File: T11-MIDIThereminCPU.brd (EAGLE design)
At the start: 102.5 x 53.3 mm, 66 parts, among them IC1 UA78M05DCY, IC4 QUAD_OPAMPD, IC5 4069D, J1 DCJ0202, Q1 16MHz, U1 ATMEGA328P-AU

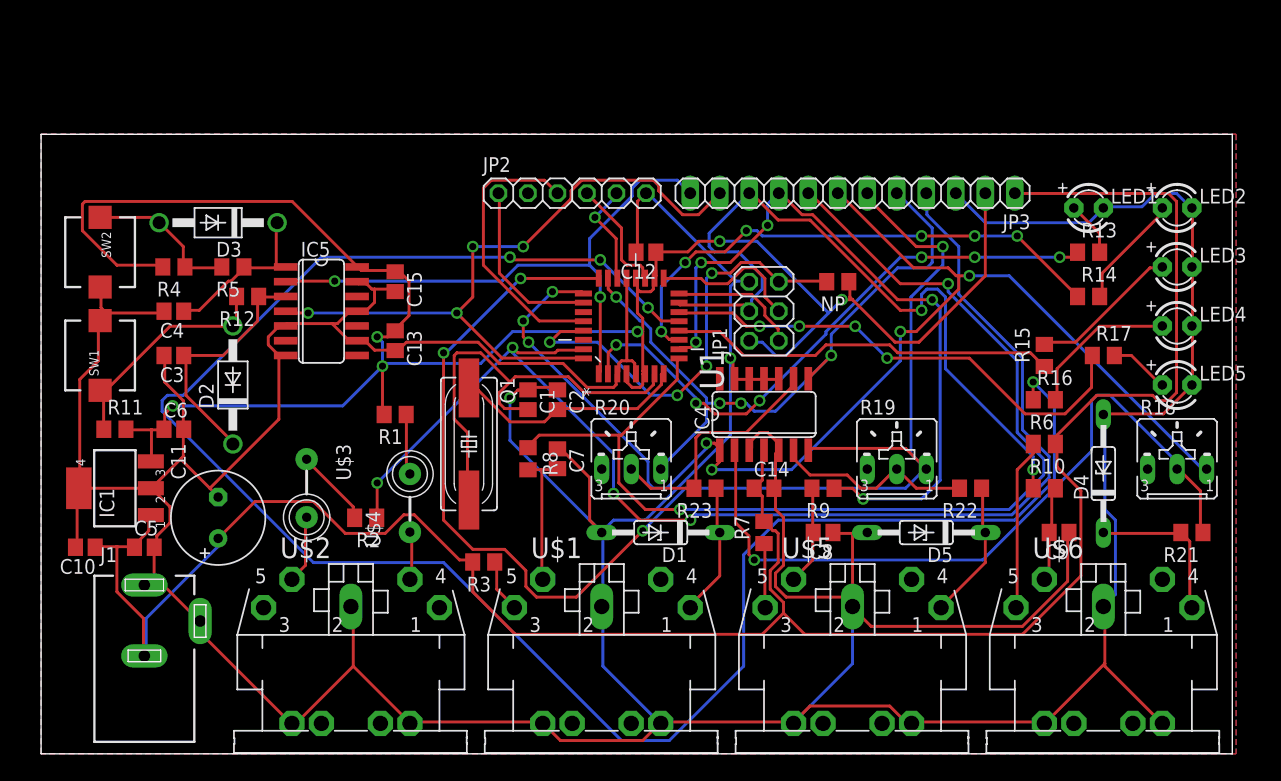
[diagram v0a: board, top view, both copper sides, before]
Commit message: Add files via upload
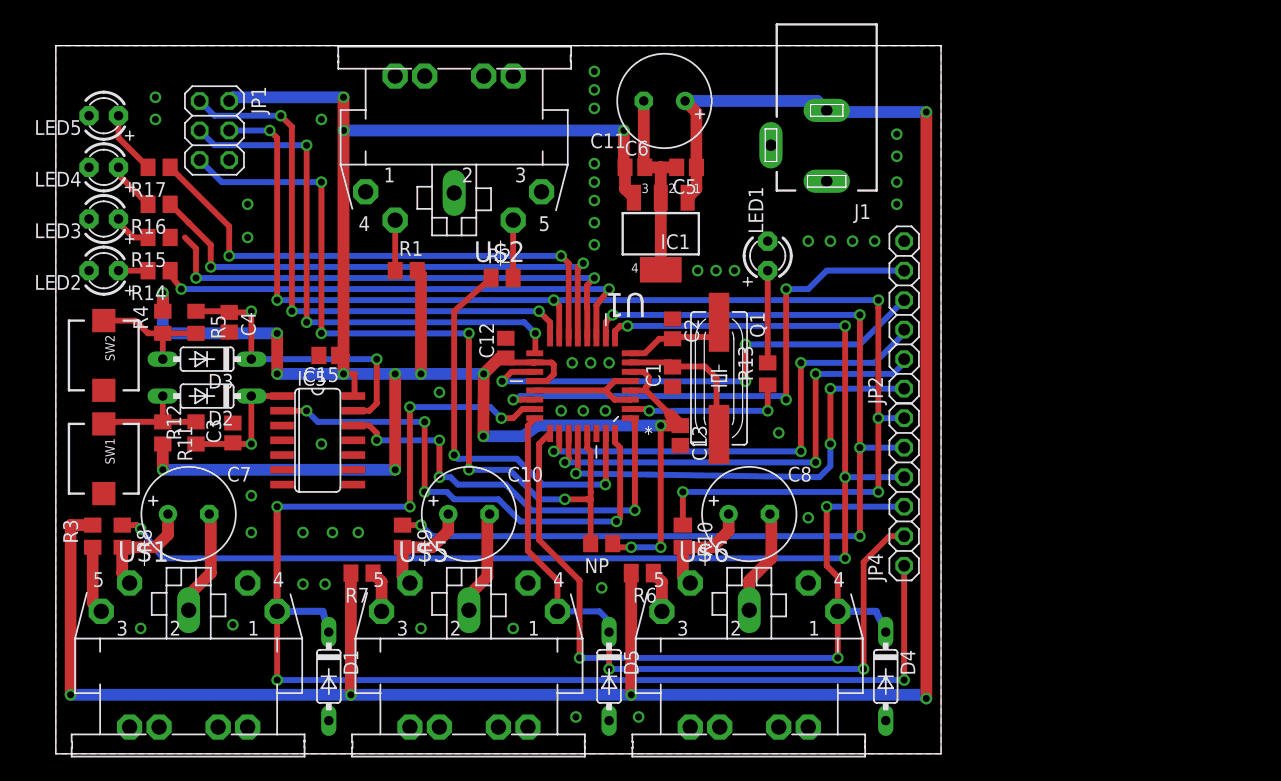
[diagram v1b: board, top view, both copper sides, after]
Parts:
- removed C14: 0.1u, adafruit:C0805
- removed C9: 100n, adafruit:C0805
- removed IC4: QUAD_OPAMPD, adafruit:SO14
- removed JP3: (no value), adafruit:1X12
- removed R18, R19, R20: 10k, pot:B25U
- removed R21, R22, R23: 1k, resistor:R0805
- removed U$3, U$4: 1k@100MHz, adafruit:FB
- added JP4: (no value), adafruit:1X06
- C10: value 0.1u -> 100uF; device adafruit:C0805 -> adafruit:E3,5-8
- C7, C8: value 100n -> 100uF; device adafruit:C0805 -> adafruit:E3,5-8
- D1, D4, D5: device diode:DO35Z10 -> diode:DO35-7
- D2, D3: value 1N4004 -> 1N4148DO35-7; device diode:DO41-10 -> diode:DO35-7
- R10, R8, R9: value 1k -> 100
- moved LED5 95.3 mm to (4.13, 54.9), turned to 180 degrees
- moved LED4 93.4 mm to (4.13, 50.5), turned to 180 degrees
- moved LED2 92.6 mm to (4.13, 41.6), turned to 180 degrees
- moved LED3 92.5 mm to (4.13, 46.0), turned to 180 degrees
- moved R17 82.9 mm to (8.89, 50.5), turned to 180 degrees
- moved R14 80.0 mm to (8.89, 41.6), turned to 180 degrees
- moved R16 78.0 mm to (8.89, 47.3), turned to 180 degrees
- moved R15 76.9 mm to (8.89, 44.5), turned to 180 degrees
- moved J1 71.6 mm to (66.4, 52.4), turned to 180 degrees
- moved U$2 61.6 mm to (34.3, 61.0), turned to 180 degrees
- moved C5 57.0 mm to (54.3, 50.5), turned to 180 degrees
- moved C11 52.6 mm to (52.4, 56.2), turned to 180 degrees
- moved IC1 51.8 mm to (52.1, 44.8), turned to 180 degrees
- moved JP1 49.8 mm to (13.7, 53.7), turned to 270 degrees
- moved C6 45.6 mm to (49.8, 50.5)
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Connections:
- removed net N$1: U$2.4, U$4.P$1
- removed net N$18: IC4.9, R20.S, R23.2
- removed net N$19: IC4.2, R18.S, R21.1
- removed net N$21: D1.C, R23.1, U$1.1
- removed net N$22: IC4.6, R19.S, R22.2
- removed net N$23: D4.C, R21.2, U$6.1
- removed net N$25: D5.C, R22.1, U$5.1
- removed net N$3: U$2.5, U$3.P$2
- net +12V: no longer C10.1, C14.1, IC4.4, JP3.1
- net +5V: no longer JP3.2
- net ANALOG_IN_1: now also D1.C, JP4.1, U$1.1; no longer IC4.8, JP3.5, R20.A
- net ANALOG_IN_2: now also D5.C, JP4.2, U$5.1; no longer IC4.7, JP3.6, R19.A
- net ANALOG_IN_3: now also D4.C, JP4.3, U$6.1; no longer IC4.1, JP3.7, R18.A
- net GND: now also C10.-, C7.-, C8.-, IC5.3; no longer C10.2, C14.2, C7.1, C8.1, C9.1, IC4.10, IC4.11, IC4.12, IC4.13, IC4.3, IC4.5, IC5.13, JP3.3
- net INT0: now also IC5.2; no longer IC5.4, JP3.11
- net INT1: now also IC5.12; no longer IC5.2, JP3.12
- net MOSI: now also JP4.6; no longer JP3.10
- net N$10: now also C10.+; no longer C8.2
- net N$13: now also U$2.5; no longer U$3.P$1
- net N$14: now also IC5.1; no longer IC5.3
- net N$2: now also U$2.4; no longer U$4.P$2
- net N$26: now also C7.+; no longer C7.2
- net N$5: now also C8.+; no longer C9.2
- net N$6: now also IC5.13; no longer IC5.1
- net PC3: now also JP2.3; no longer JP2.1
- net PC5: now also JP2.1; no longer JP2.3
- net SIGNAL_OUT_1: now also JP4.4; no longer JP3.8
- net SIGNAL_OUT_2: now also JP4.5; no longer JP3.9
- net TX: no longer JP3.4
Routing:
- net GND: track 485.2 -> 56.4 mm, vias 2 -> 48
- net LED_4: track 167.0 -> 46.4 mm, vias 4 -> 2
- net TX: track 110.8 -> 35.1 mm, vias 4 -> 2
- net N$19: track 64.4 -> 0.00 mm, vias 1 -> 0
- net ANALOG_IN_2: track 120.5 -> 62.4 mm, vias 4 -> 2
- net ANALOG_IN_1: track 57.9 -> 116.0 mm, vias 4 -> 6
- net MOSI: track 64.1 -> 112.0 mm, vias 2 -> 7
- net PC4: track 0.00 -> 40.2 mm, vias 0 -> 3
- net ANALOG_IN_3: track 107.2 -> 68.8 mm, vias 7 -> 3
- net MISO: track 11.2 -> 48.7 mm, vias 0 -> 3
- net LED_1: track 51.1 -> 14.1 mm, vias 6 -> 2
- net ADC7: track 9.13 -> 45.9 mm, vias 1 -> 3
- net SCK: track 13.2 -> 46.8 mm, vias 0 -> 3
- net ADC6: track 10.1 -> 42.5 mm, vias 0 -> 3
- net RST: track 38.9 -> 69.9 mm, vias 4 -> 5
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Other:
- board size 102.5 x 53.3 mm -> 76.2 x 61 mm
